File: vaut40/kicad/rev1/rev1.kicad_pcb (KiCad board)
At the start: 2 copper layers, 228.3 x 128.1 mm, 90 parts, among them SW1 SW_PUSH, SW10 SW_PUSH, SW11 SW_PUSH, SW12 SW_PUSH, SW13 SW_PUSH, SW14 SW_PUSH, SW15 SW_PUSH, SW16 SW_PUSH, SW17 SW_PUSH, SW18 SW_PUSH, SW19 SW_PUSH, SW2 SW_PUSH, SW20 SW_PUSH, SW21 SW_PUSH, SW22 SW_PUSH, SW23 SW_PUSH, SW24 SW_PUSH, SW25 SW_PUSH, SW26 SW_PUSH, SW27 SW_PUSH, SW28 SW_PUSH, SW29 SW_PUSH, SW3 SW_PUSH, SW30 SW_PUSH, SW31 SW_PUSH, SW32 SW_PUSH, SW33 SW_PUSH, SW34 SW_PUSH, SW35 SW_PUSH, SW36 SW_PUSH, SW37 SW_PUSH, SW38 SW_PUSH, SW39 SW_PUSH, SW4 SW_PUSH, SW40 SW_PUSH, SW41 SW_PUSH, SW5 SW_PUSH, SW6 SW_PUSH, SW7 SW_PUSH, SW8 SW_PUSH, SW9 SW_PUSH, U1 ProMicro_r

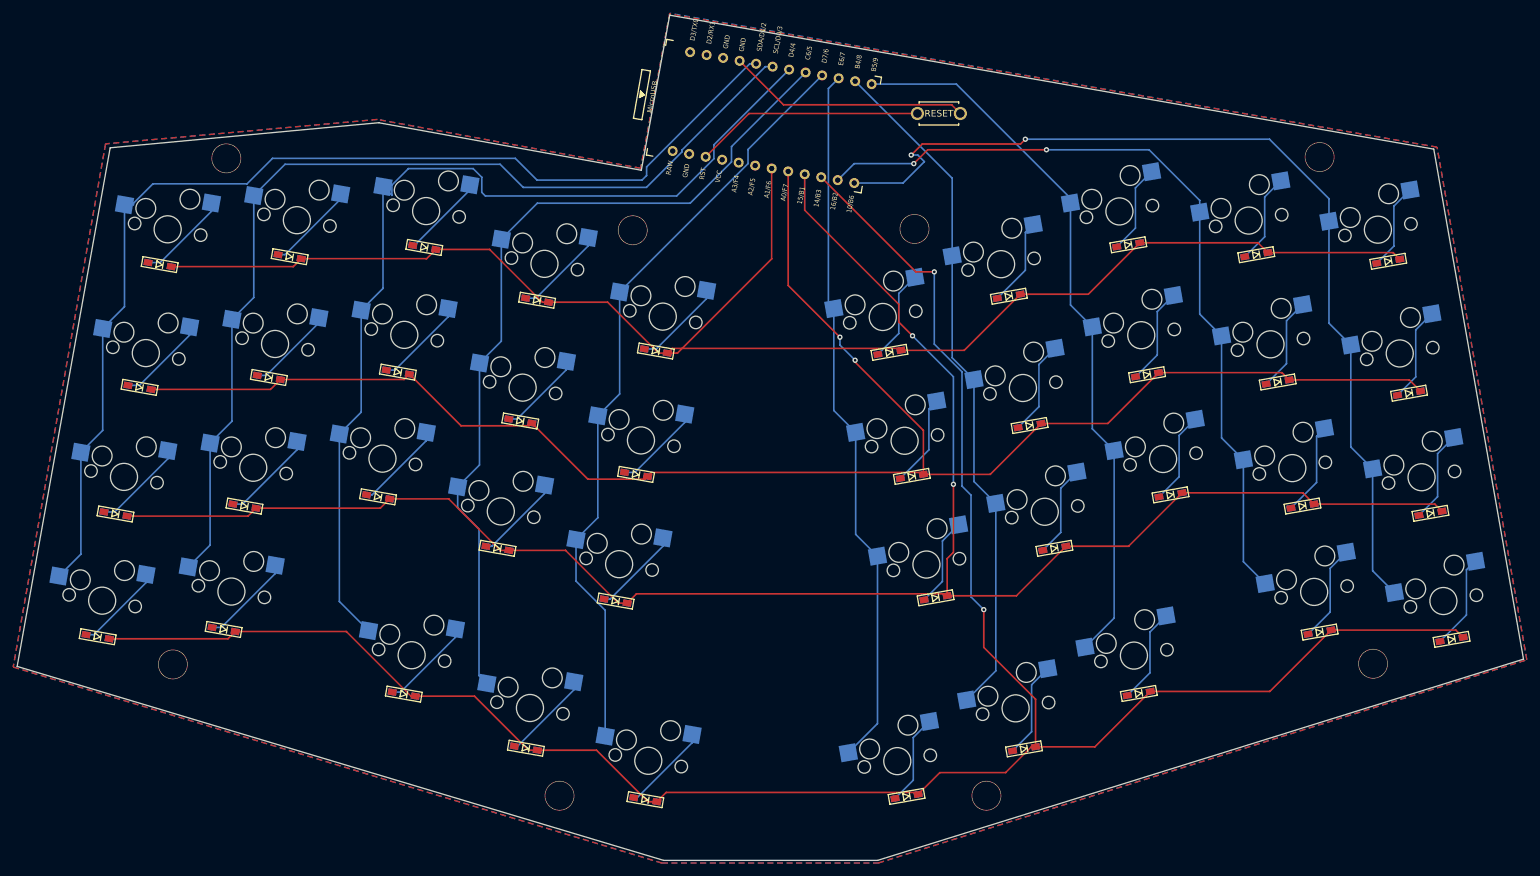
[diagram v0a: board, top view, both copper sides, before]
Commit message: fix error of pcb
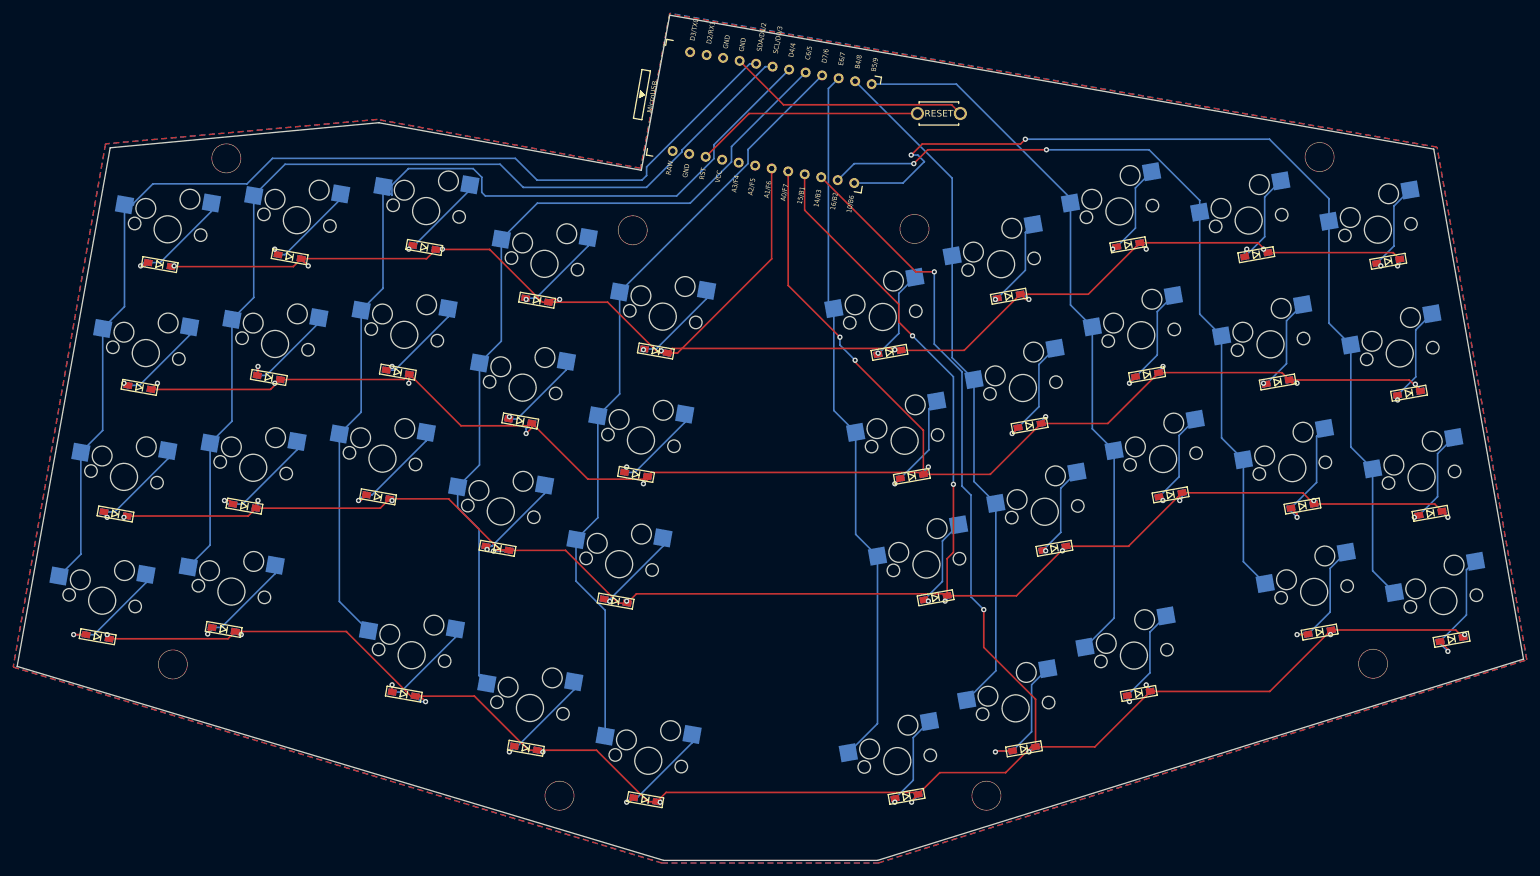
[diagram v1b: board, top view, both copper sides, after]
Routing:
- net Row1: track 262.8 -> 290.5 mm, vias 2 -> 12
- net Row0: track 237.4 -> 261.3 mm, vias 0 -> 10
- net Row3: track 329.2 -> 350.5 mm, vias 2 -> 12
- net Row2: track 288.9 -> 308.9 mm, vias 2 -> 12
- net Net-(D37-A): track 14.7 -> 20.0 mm, vias 0 -> 1
- net Net-(D40-A): track 14.4 -> 18.4 mm, vias 0 -> 1
- net Net-(D31-A): track 13.6 -> 17.4 mm, vias 0 -> 1
- net Net-(D29-A): track 14.2 -> 17.7 mm, vias 0 -> 1
- net Net-(D39-A): track 14.8 -> 18.2 mm, vias 0 -> 1
- net Net-(D23-A): track 13.7 -> 16.9 mm, vias 0 -> 1
- net Net-(D22-A): track 14.4 -> 17.4 mm, vias 0 -> 1
- net Net-(D12-A): track 13.4 -> 16.2 mm, vias 0 -> 1
- net Net-(D18-A): track 14.7 -> 17.4 mm, vias 0 -> 1
- net Net-(D35-A): track 13.5 -> 16.3 mm, vias 0 -> 1
- net Net-(D1-A): track 14.1 -> 16.8 mm, vias 0 -> 1
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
